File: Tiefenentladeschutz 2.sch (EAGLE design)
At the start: 38 parts, among them IC1 ICL7665CSA, IC2 NE555D

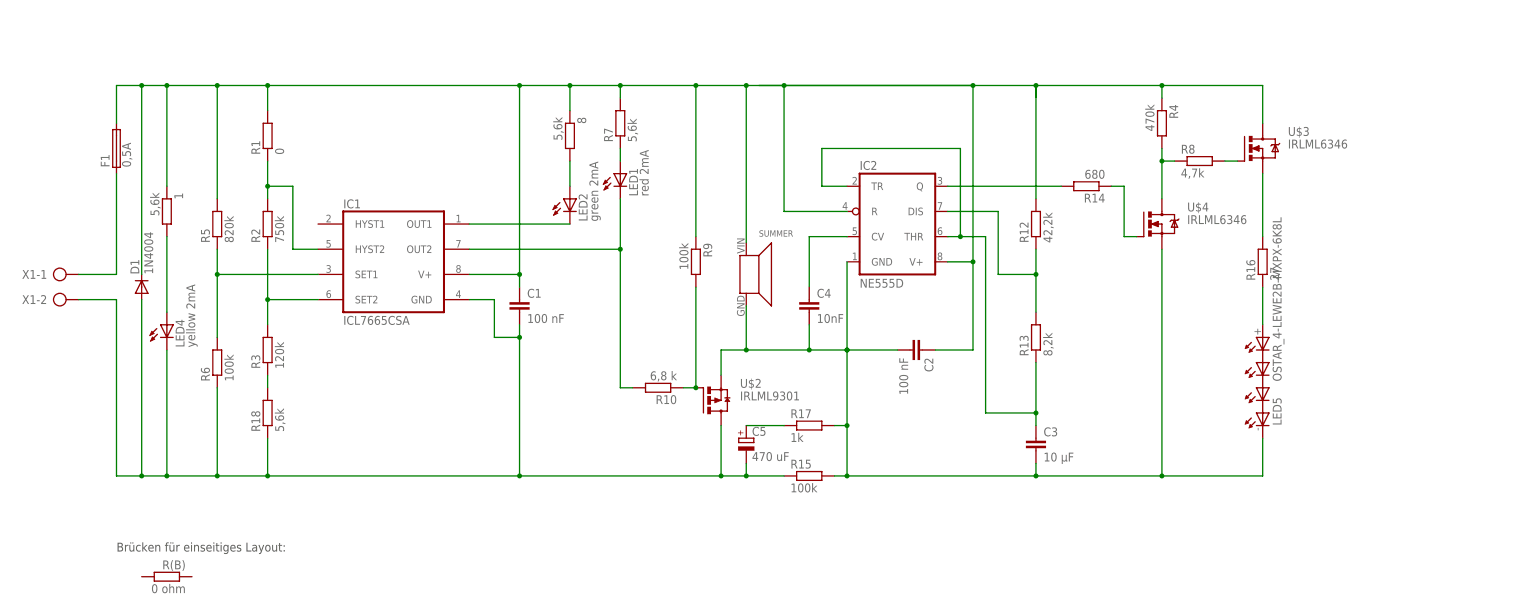
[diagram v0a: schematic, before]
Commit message: 3.0
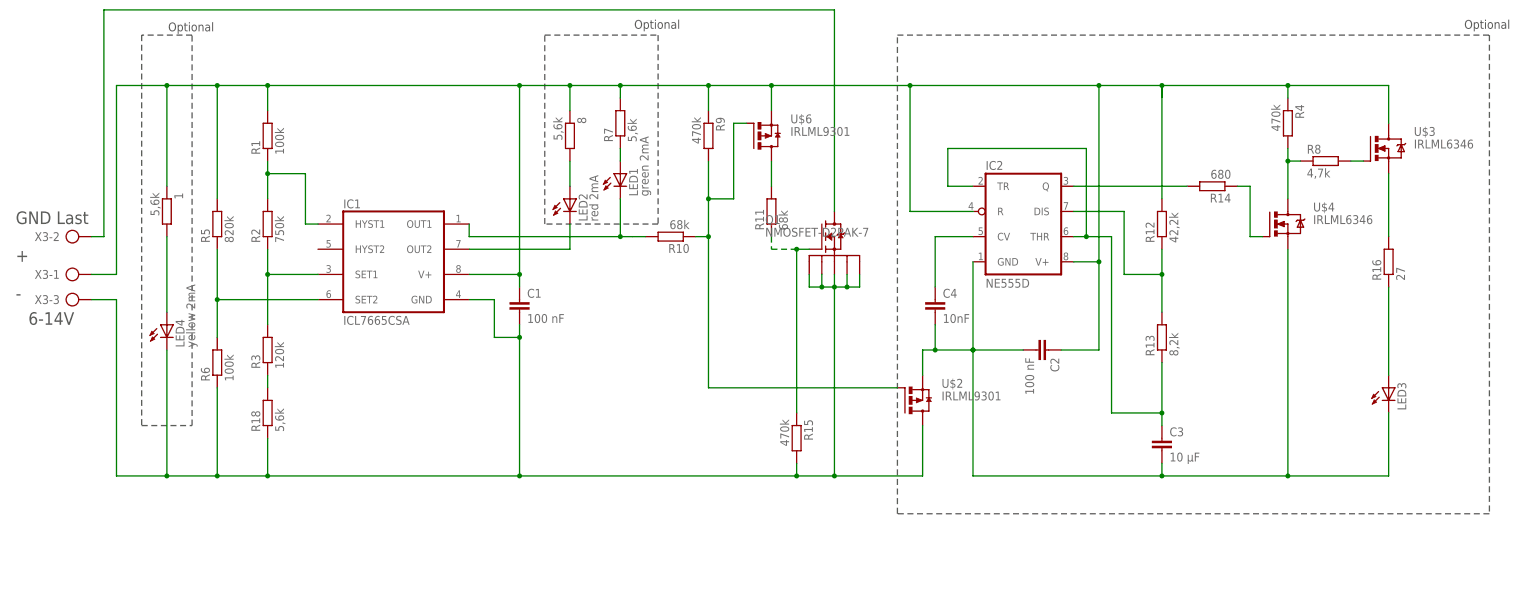
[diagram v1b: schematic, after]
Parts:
- removed C5: 470 uF, rcl:CPOL-EUTT5D10
- removed D1: 1N4004, diode:1N4004
- removed F1: 0,5A, fuse:FUSESH22,5A
- removed LED5: OSTAR_4-LEWE2B-MXPX-6K8L, led:OSTAR_4-LEWE2B-MXPX-6K8L
- removed R(B): 0 ohm, eagle-ltspice:RR1206
- removed R17: 1k, eagle-ltspice:RR1206
- removed SUMMER: SUMMER3, 0liver:SUMMER3
- removed X1: (no value), con-ptr500:AK300/2
- added LED3: (no value), led:LEDP-LCC-2
- added Q1: NMOSFET-D2PAK-7, D2pak-7:NMOSFET-D2PAK-7
- added R11: 68k, eagle-ltspice:RR1206
- added U$6: IRLML9301, 0liver:IRLML9301
- added X3: (no value), con-ptr500:AK500/3
- C1: device eagle-ltspice:CC0603 -> eagle-ltspice:CC1206
- LED1: value red 2mA -> green 2mA
- LED2: value green 2mA -> red 2mA
- R1: value 0 -> 100k
- R10: value 6,8 k -> 68k
- R15, R9: value 100k -> 470k
- R16: device resistor:R-EU_0617/17 -> resistor:R-EU_0414/15
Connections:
- removed net N$23: C5.+, R17.1
- removed net POWER-IN: F1.1, X1-1.KL
- new net N$13: IC1.HYST1, R1.1, R2.2
- new net N$16: IC1.OUT1, LED1.C, R10.2
- new net N$22: Q1.G, R11.1, R15.1
- net 2NDGND: now also LED3.C; no longer LED5.C, R15.2, R17.2, SUMMER.-
- net GND: now also Q1.S1, Q1.S2, Q1.S3, Q1.S4, Q1.S5, R15.2, X3-3.KL; no longer C5.-, D1.A, R15.1, X1-2.KL
- net N$1: now also Q1.D, X3-2.KL; no longer IC1.HYST2, R1.1, R2.2
- net N$10: now also R11.2, U$6.D; no longer IC1.OUT2, LED1.C, R10.2
- net N$11: now also IC1.OUT2; no longer IC1.OUT1
- net N$12: now also LED3.A; no longer LED5.A
- net N$2: now also IC1.SET1; no longer IC1.SET2
- net N$4: now also IC1.SET2; no longer IC1.SET1
- net N$7: now also U$6.G
- net V+: now also U$6.S, X3-1.KL; no longer D1.C, F1.2, SUMMER.+
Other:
- note added: "+"
- note added: "-"
- note added: "6-14V"
- note added: "GND Last"
- note added: "Optional"
- note removed: "Brücken für einseitiges Layout:"
- moved on the sheet: C2, C3, C4, IC2, R10, R12, R13, R14, R15, R16, R4, R8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

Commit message: 3.3
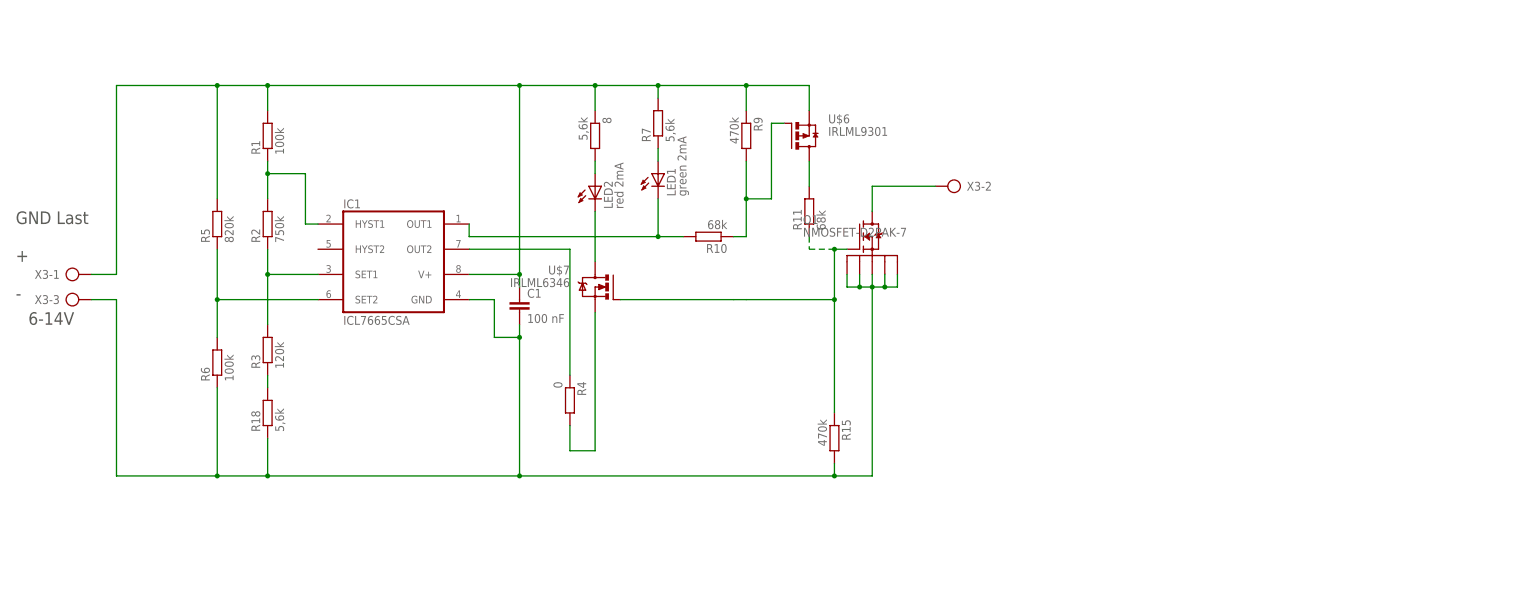
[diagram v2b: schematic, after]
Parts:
- removed 1: 5,6k, eagle-ltspice:RR1206
- removed C2: 100 nF, eagle-ltspice:CC0603
- removed C3: 10 µF, eagle-ltspice:CC1206
- removed C4: 10nF, rcl:C-EUC0805K
- removed IC2: NE555D, linear:NE555D
- removed LED3: (no value), led:LEDP-LCC-2
- removed LED4: yellow 2mA, eagle-ltspice:LED_ESML0603
- removed R12: 42,2k, eagle-ltspice:RR1206
- removed R13: 8,2k, eagle-ltspice:RR1206
- removed R14: 680, eagle-ltspice:RR1206
- removed R16: 27, resistor:R-EU_0414/15
- removed R8: 4,7k, eagle-ltspice:RR1206
- removed U$2: IRLML9301, 0liver:IRLML9301
- removed U$3, U$4: IRLML6346, 0liver:IRLML6346
- added U$7: IRLML6346, 0liver:IRLML6346
- R4: value 470k -> 0
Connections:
- removed net 2NDGND: C2.2, C3.2, C4.2, IC2.GND, LED3.C, U$2.S, U$4.S
- removed net N$12: LED3.A, R16.1
- removed net N$15: IC2.DIS, R12.1, R13.2
- removed net N$17: R8.2, U$3.G
- removed net N$18: R14.1, U$4.G
- removed net N$19: C4.1, IC2.CV
- removed net N$20: C3.1, IC2.THR, IC2.TR, R13.1
- removed net N$21: R4.2, R8.1, U$4.D
- removed net N$8: IC2.Q, R14.2
- removed net N$9: 1.2, LED4.A
- new net N$23: IC1.OUT2, R4.1
- net GND: no longer LED4.C, U$2.D
- net N$11: now also U$7.D; no longer IC1.OUT2
- net N$22: now also U$7.G
- net N$3: now also R4.2, U$7.S; no longer R16.2, U$3.S
- net N$7: no longer U$2.G
- net V+: no longer 1.1, C2.1, IC2.R, IC2.V+, R12.2, R4.1, U$3.D
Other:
- note removed: "Optional"
- moved on the sheet: 8, LED1, LED2, Q1, R10, R11, R15, R4, R7, R9, U$6, X3-2

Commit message: 3.5
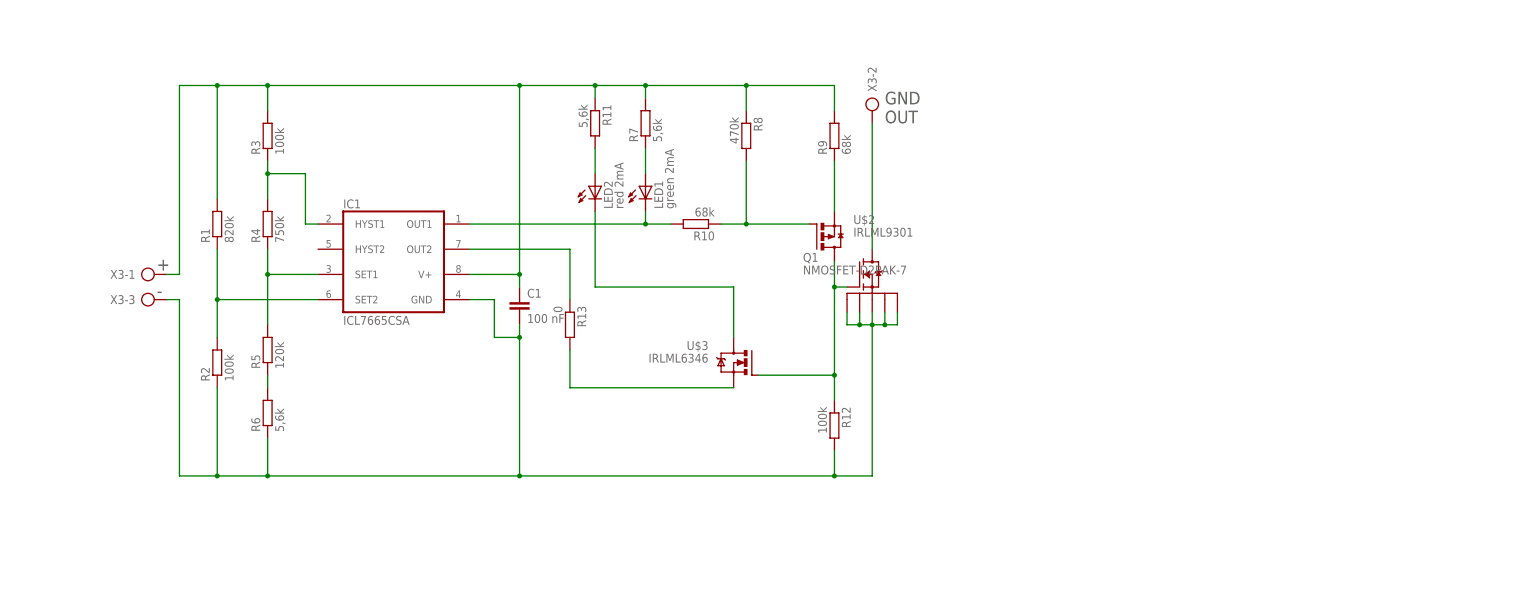
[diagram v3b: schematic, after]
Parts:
- removed 8, R18: 5,6k, eagle-ltspice:RR1206
- removed R15: 470k, eagle-ltspice:RR1206
- removed U$6: IRLML9301, 0liver:IRLML9301
- removed U$7: IRLML6346, 0liver:IRLML6346
- added R12: 100k, eagle-ltspice:RR1206
- added R13: 0, eagle-ltspice:RR1206
- added R8: 470k, eagle-ltspice:RR1206
- added U$2: IRLML9301, 0liver:IRLML9301
- added U$3: IRLML6346, 0liver:IRLML6346
- R1: value 100k -> 820k
- R11: value 68k -> 5,6k
- R2: value 750k -> 100k
- R3: value 120k -> 100k
- R4: value 0 -> 750k
- R5: value 820k -> 120k
- R6: value 100k -> 5,6k
- R9: value 470k -> 68k
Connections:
- removed net N$10: R11.2, U$6.D
- new net N$8: R9.1, U$2.S
- net GND: now also R12.2, R2.1; no longer R15.2, R18.1
- net N$11: now also U$3.D; no longer U$7.D
- net N$13: now also R3.1, R4.2; no longer R1.1, R2.2
- net N$2: now also R4.1, R5.2; no longer R2.1, R3.2
- net N$22: now also R12.1, U$2.D, U$3.G; no longer R11.1, R15.1, U$7.G
- net N$23: now also R13.1; no longer R4.1
- net N$26: now also R5.1, R6.2; no longer R18.2, R3.1
- net N$3: now also R13.2, U$3.S; no longer R4.2, U$7.S
- net N$4: now also R1.1, R2.2; no longer R5.1, R6.2
- net N$5: now also R11.2; no longer 8.2
- net N$7: now also R8.2, U$2.G; no longer R9.2, U$6.G
- net V+: now also R11.1, R3.2, R8.1, R9.2; no longer 8.1, R5.2, R9.1, U$6.S
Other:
- note added: "GND OUT"
- note removed: "6-14V"
- note removed: "GND Last"
- moved on the sheet: LED1, Q1, R1, R10, R11, R2, R3, R4, R5, R6, R7, R9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

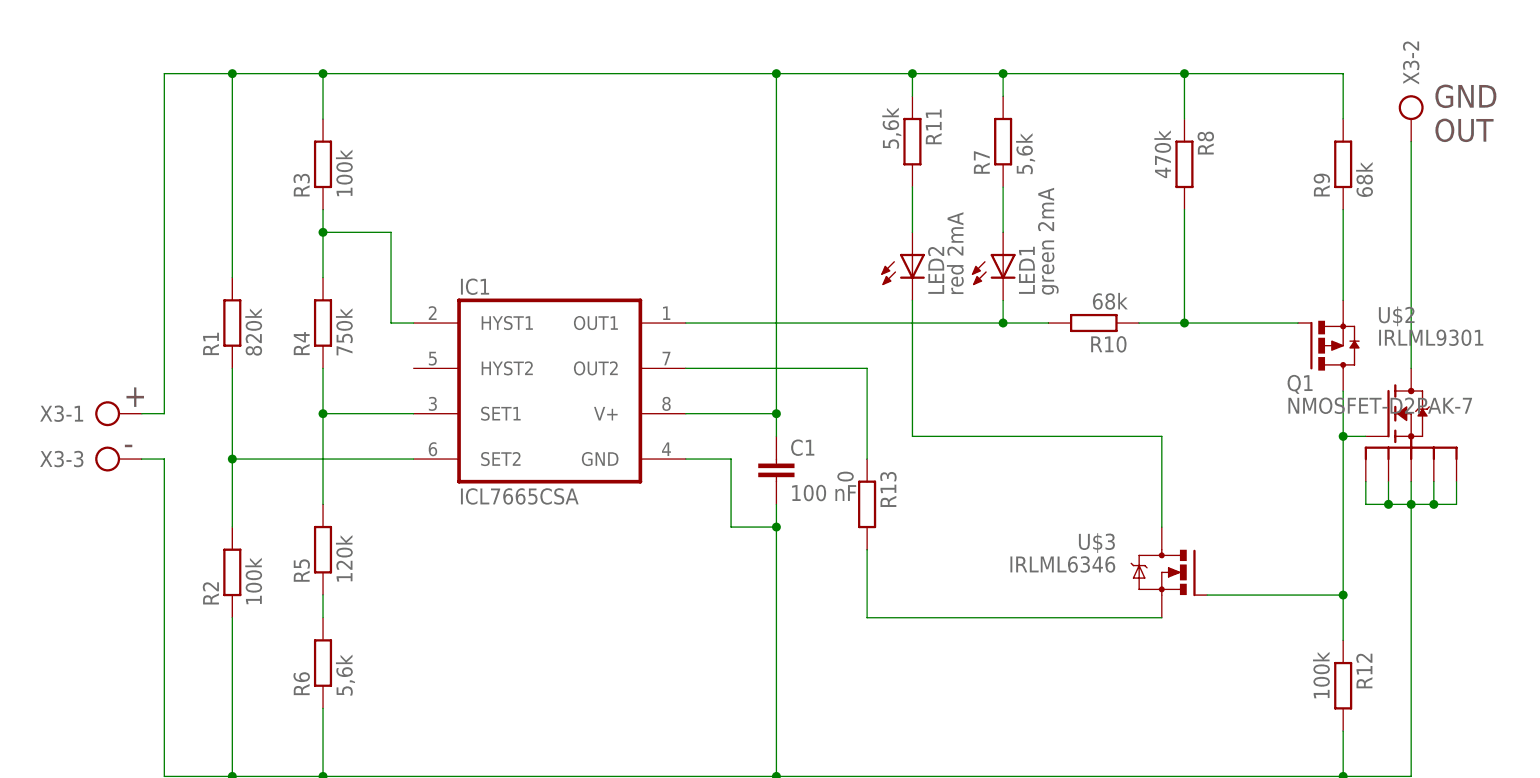
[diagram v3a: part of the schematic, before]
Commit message: 3.7
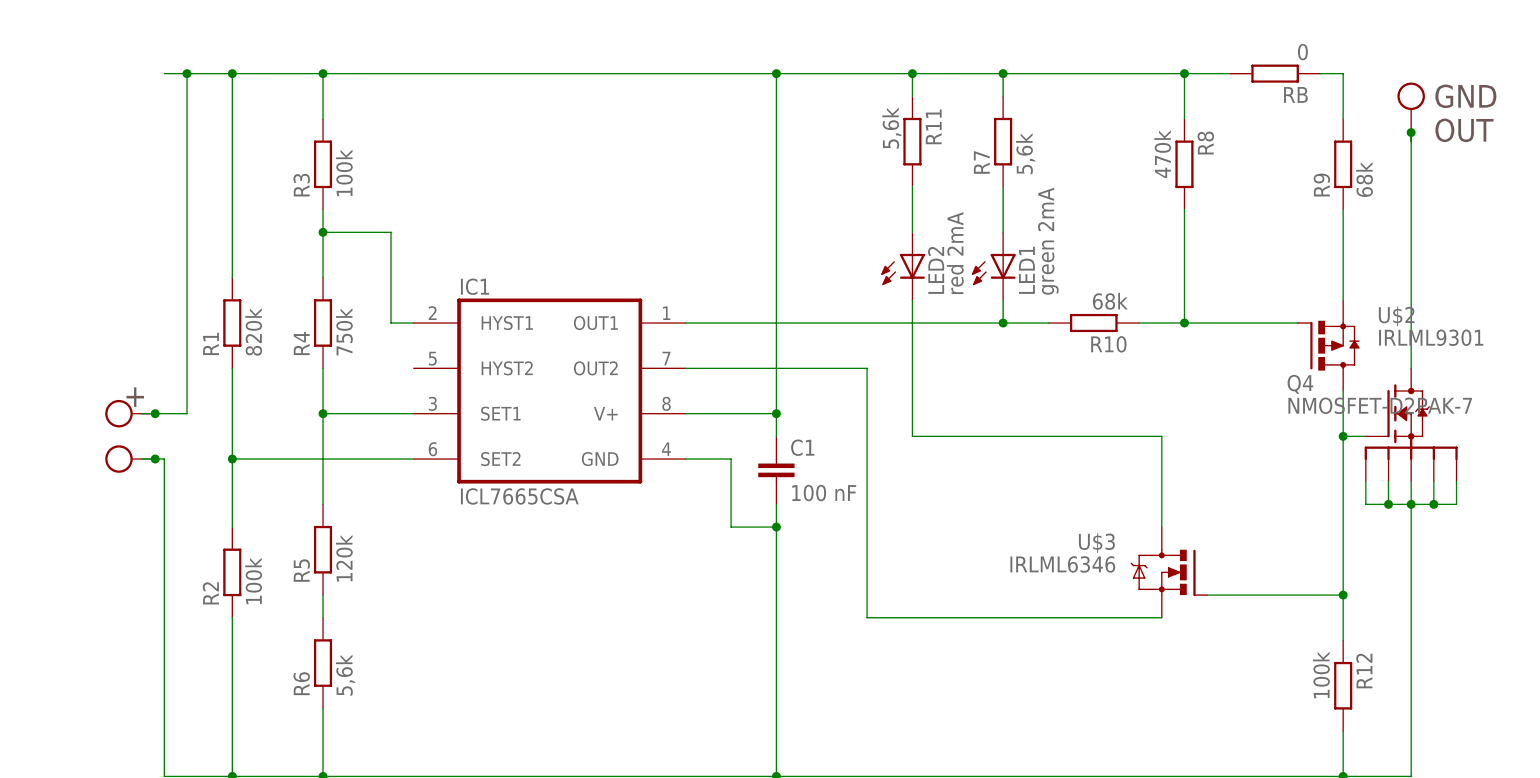
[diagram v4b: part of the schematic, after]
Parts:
- removed R13: 0, eagle-ltspice:RR1206
- removed X3: (no value), con-ptr500:AK500/3
- added RB: 0, eagle-ltspice:RR1206
- added U$4: (no value), 0liver:PINBIG
- added U$6, U$7: (no value), 0liver:PIN1.27
- renumbered Q1 to Q4
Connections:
- removed net N$23: IC1.OUT2, R13.1
- new net N$10: R9.2, RB.1
- net GND: now also U$6.P$1; no longer X3-3.KL
- net N$1: now also U$7.P$1; no longer X3-2.KL
- net N$3: now also IC1.OUT2; no longer R13.2
- net V+: now also RB.2, U$4.P$1; no longer R9.2, X3-1.KL
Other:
- note removed: "-"
